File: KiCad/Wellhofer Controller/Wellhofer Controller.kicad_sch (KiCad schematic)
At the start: 13 parts, among them Q1 PMOS, Q10 NMOS, Q11 PMOS, Q12 NMOS, Q2 NMOS, Q3 PMOS, Q4 NMOS, Q5 PMOS, Q6 NMOS, Q7 PMOS, Q8 NMOS, Q9 PMOS

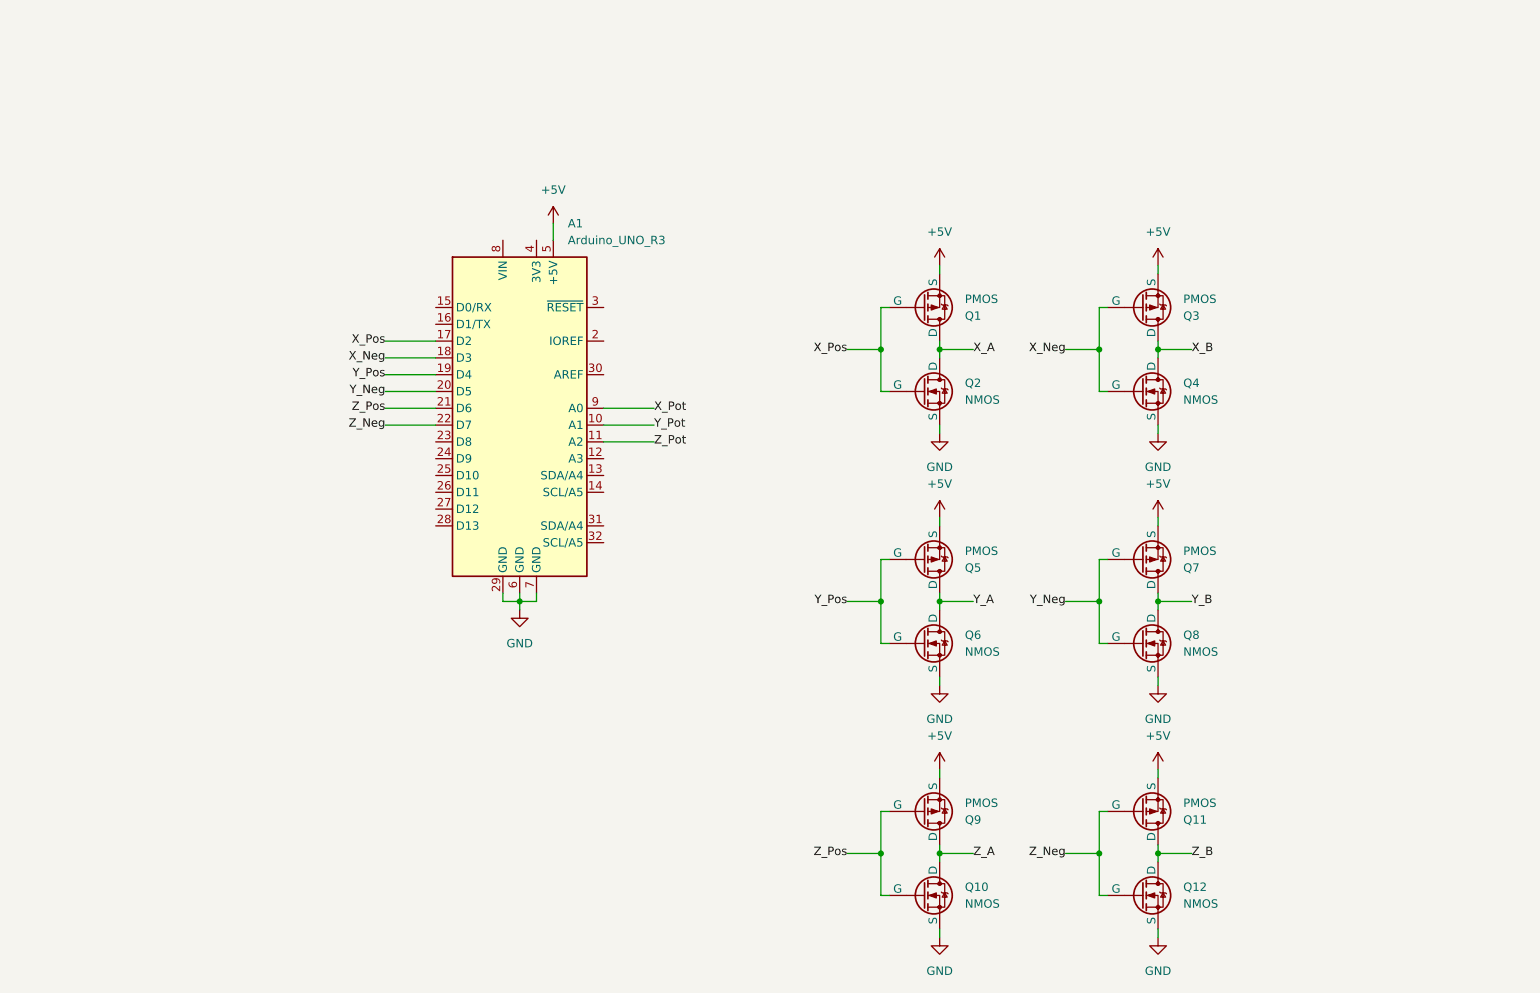
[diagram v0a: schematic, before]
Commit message: Final schematic
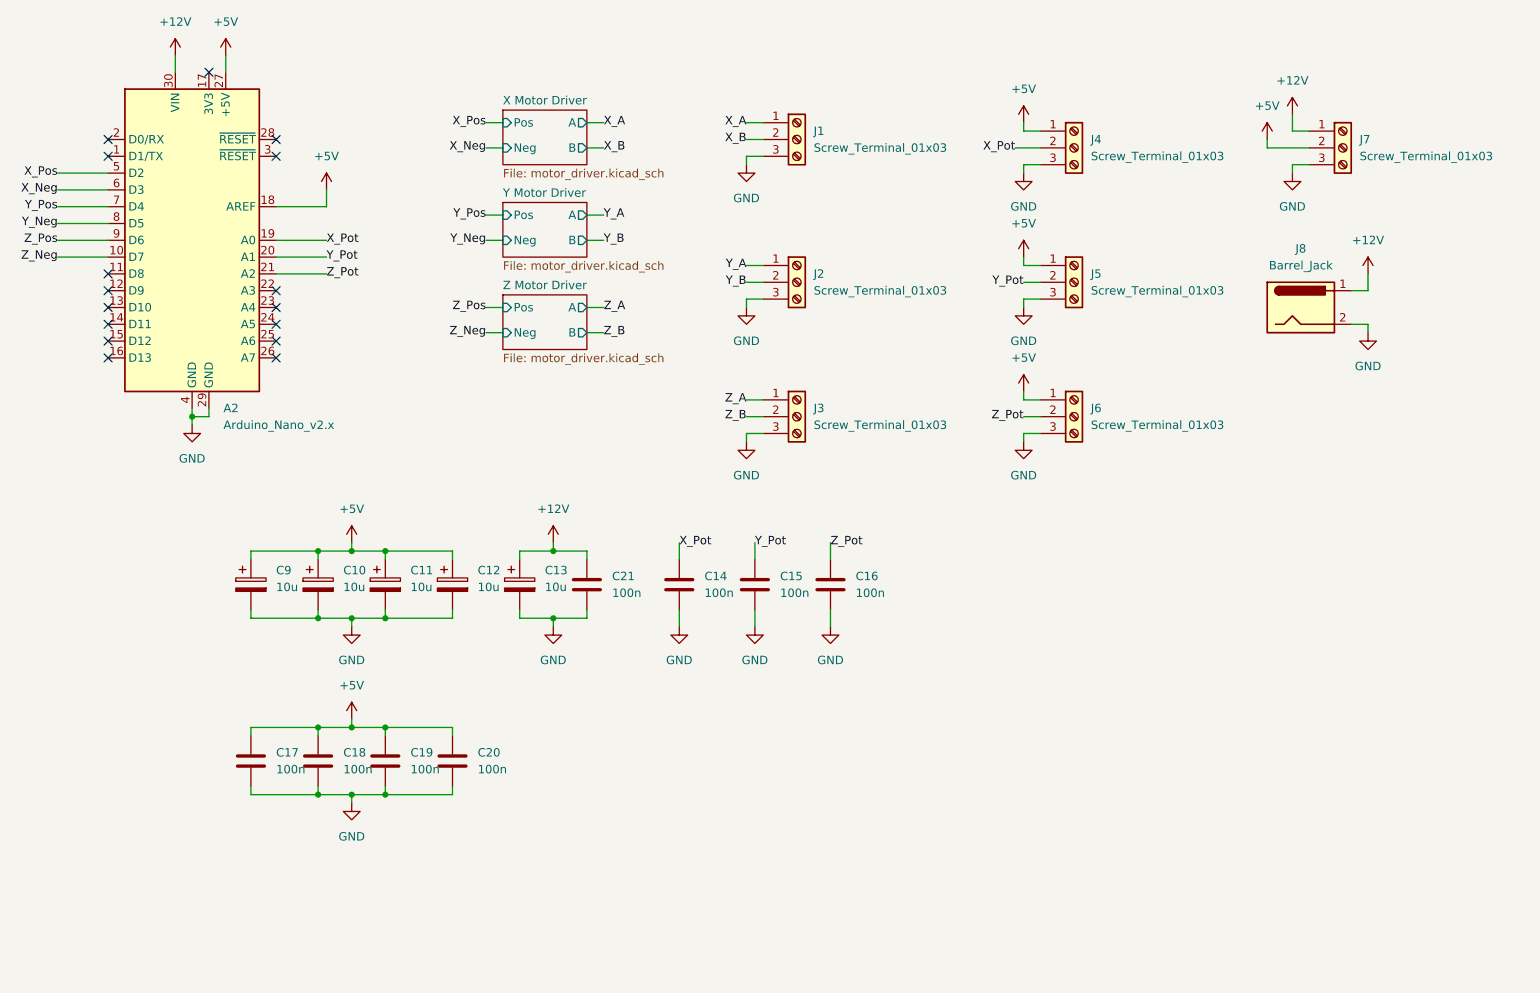
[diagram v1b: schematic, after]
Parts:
- removed A1: Arduino_UNO_R3, Module:Arduino_UNO_R3, symbol MCU_Module:Arduino_UNO_R3
- removed Q1, Q11, Q3, Q5, Q7, Q9: PMOS, symbol Simulation_SPICE:PMOS
- removed Q10, Q12, Q2, Q4, Q6, Q8: NMOS, symbol Simulation_SPICE:NMOS
- added A2: Arduino_Nano_v2.x, Module:Arduino_Nano, symbol MCU_Module:Arduino_Nano_v2.x
- added C10, C11, C12, C13, C9: 10u, symbol Device:C_Polarized
- added C14, C15, C16, C17, C18, C19, C20, C21: 100n, symbol Device:C
- added J1, J2, J3, J4, J5, J6, J7: Screw_Terminal_01x03, symbol Connector:Screw_Terminal_01x03
- added J8: Barrel_Jack, symbol Connector:Barrel_Jack
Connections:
- net +5V: now also A2.18 (AREF), A2.27 (+5V), C10.1, C11.1, C12.1, C17.1, C18.1, C19.1, C20.1, C9.1, J4.1 (Pin_1), J5.1 (Pin_1), J6.1 (Pin_1), J7.2 (Pin_2)
- net GND: now also A2.29 (GND), A2.4 (GND), C10.2, C11.2, C12.2, C13.2, C14.2, C15.2, C16.2, C17.2, C18.2, C19.2, C20.2, C21.2, C9.2, J1.3 (Pin_3), J2.3 (Pin_3), J3.3 (Pin_3), J4.3 (Pin_3), J5.3 (Pin_3), J6.3 (Pin_3), J7.3 (Pin_3), J8.2
- net X_A: now also J1.1 (Pin_1)
- net X_B: now also J1.2 (Pin_2)
- net X_Neg: now also A2.6 (D3)
- net X_Pos: now also A2.5 (D2)
- net X_Pot: now also A2.19 (A0), C14.1, J4.2 (Pin_2)
- net Y_A: now also J2.1 (Pin_1)
- net Y_B: now also J2.2 (Pin_2)
- net Y_Neg: now also A2.8 (D5)
- net Y_Pos: now also A2.7 (D4)
- net Y_Pot: now also A2.20 (A1), C15.1, J5.2 (Pin_2)
- net Z_A: now also J3.1 (Pin_1)
- net Z_B: now also J3.2 (Pin_2)
- net Z_Neg: now also A2.10 (D7)
- net Z_Pos: now also A2.9 (D6)
- net Z_Pot: now also A2.21 (A2), C16.1, J6.2 (Pin_2)
- new net +12V: A2.30 (VIN), C13.1, C21.1, J7.1 (Pin_1), J8.1
- no-connect marks 0 -> 16
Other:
- added sheet X Motor Driver (motor_driver.kicad_sch)
- added sheet Y Motor Driver (motor_driver.kicad_sch)
- added sheet Z Motor Driver (motor_driver.kicad_sch)
